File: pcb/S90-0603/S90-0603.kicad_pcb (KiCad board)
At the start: 2 copper layers, 100 x 40 mm, 9 parts

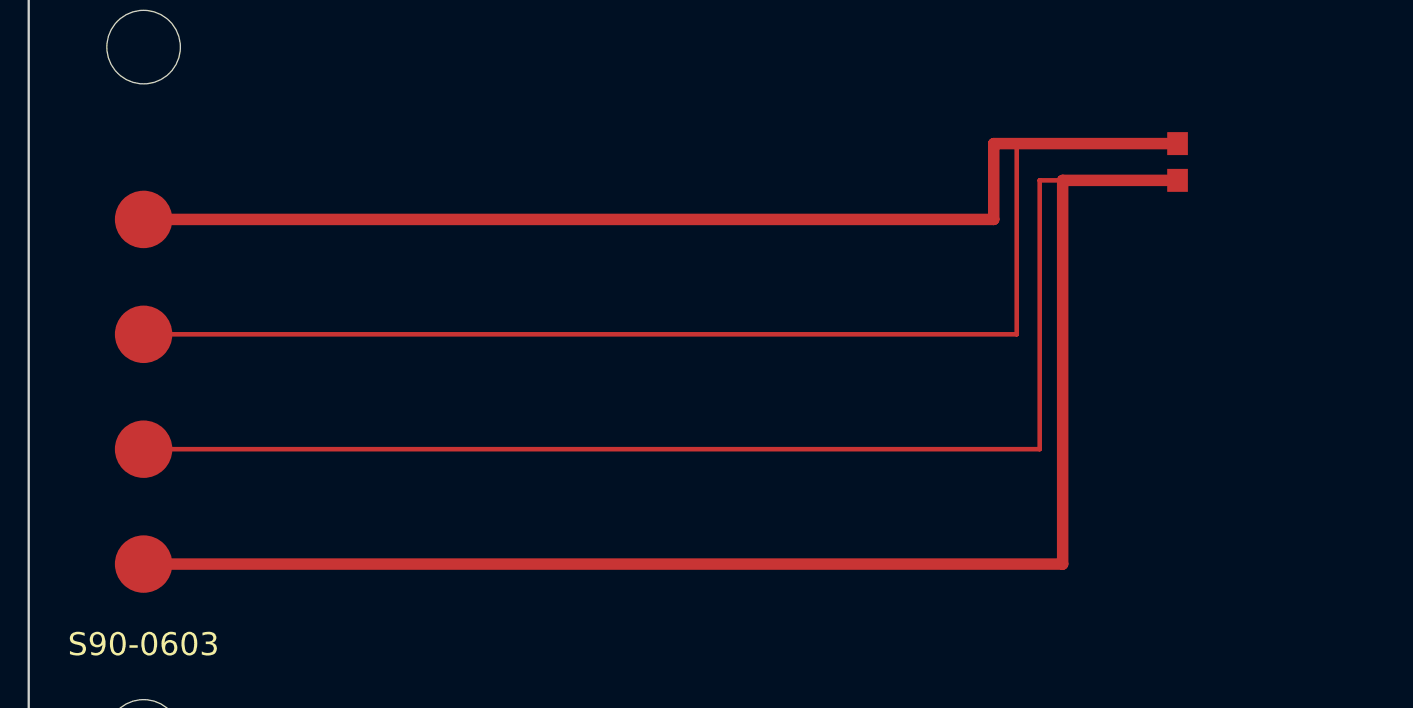
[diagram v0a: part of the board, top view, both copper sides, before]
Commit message: v0.3.1 — PCB CAD & JLCPCB Fabrication Package
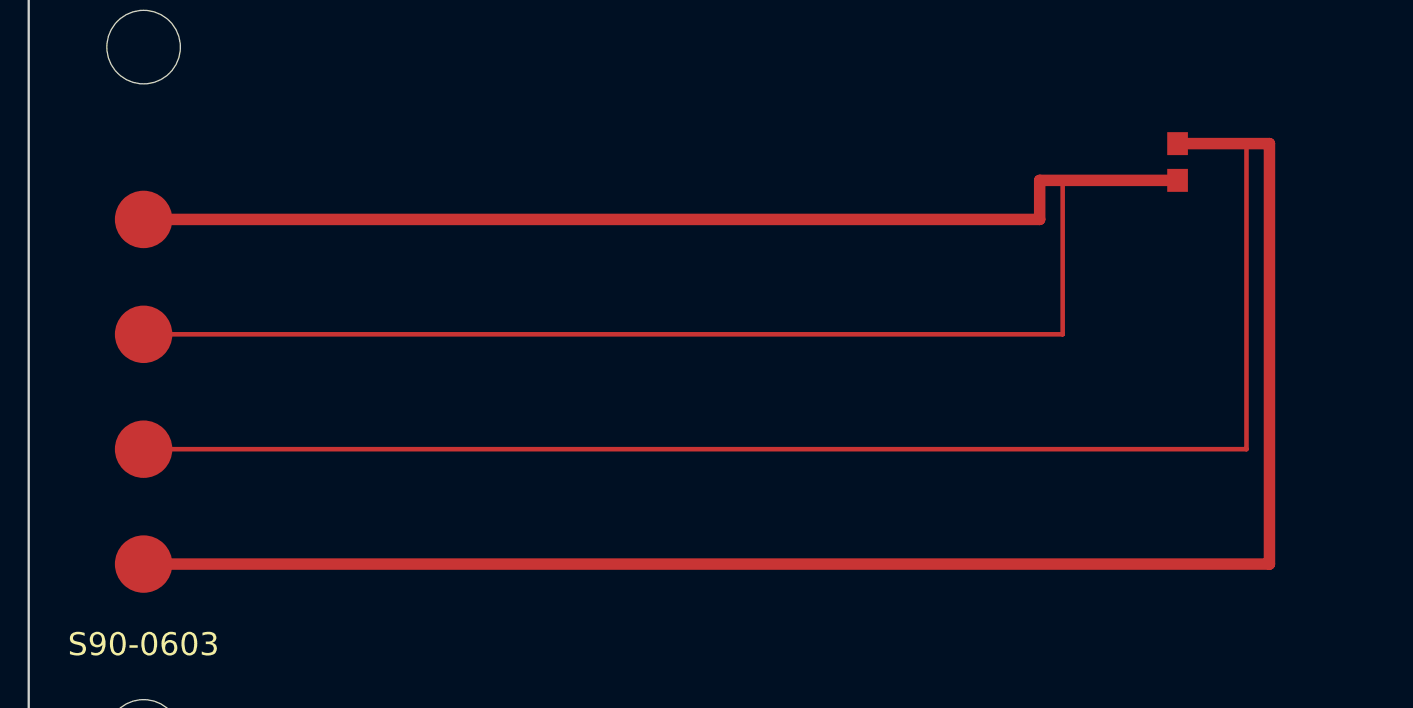
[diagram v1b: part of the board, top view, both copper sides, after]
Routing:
- net DRIVE_SENSE_MINUS: track 118.4 -> 135.6 mm
- net DRIVE_SENSE_PLUS: track 101.6 -> 98.4 mm
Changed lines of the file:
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@@
 		(pad "1" smd rect (at -0.8 0) (size 0.9 1.0) (layers "F.Cu" "F.Paste" "F.Mask") (net 1 "DRIVE_SENSE_PLUS"))
 		(pad "2" smd rect (at 0.8 0) (size 0.9 1.0) (layers "F.Cu" "F.Paste" "F.Mask") (net 2 "DRIVE_SENSE_MINUS"))
+		(model "/Applications/KiCad/KiCad.app/Contents/SharedSupport/3dmodels/Capacitor_SMD.3dshapes/C_0603_1608Metric.step"
+			(offset (xyz 0 0 0))
+			(scale (xyz 1 1 1))
+			(rotate (xyz 0 0 0))
+		)
 	)
 	(footprint "SC4:EdgeContact_2.5mm_Round" (layer "F.Cu")
@@
 		(pad "1" smd circle (at 0 0) (size 2.5 2.5) (layers "F.Cu" "F.Mask") (net 2 "DRIVE_SENSE_MINUS"))
 	)
-	(segment (start 5.0 12.5) (end 42.0 12.5) (width 0.5) (layer "F.Cu") (net 1))
-	(segment (start 42.0 12.5) (end 42.0 9.2) (width 0.5) (layer "F.Cu") (net 1))
-	(segment (start 42.0 9.2) (end 50.0 9.2) (width 0.5) (layer "F.Cu") (net 1))
-	(segment (start 5.0 17.5) (end 43.0 17.5) (width 0.2) (layer "F.Cu") (net 1))
-	(segment (start 43.0 17.5) (end 43.0 9.2) (width 0.2) (layer "F.Cu") (net 1))
-	(segment (start 43.0 9.2) (end 50.0 9.2) (width 0.2) (layer "F.Cu") (net 1))
-	(segment (start 5.0 22.5) (end 44.0 22.5) (width 0.2) (layer "F.Cu") (net 2))
-	(segment (start 44.0 22.5) (end 44.0 10.8) (width 0.2) (layer "F.Cu") (net 2))
-	(segment (start 44.0 10.8) (end 50.0 10.8) (width 0.2) (layer "F.Cu") (net 2))
-	(segment (start 5.0 27.5) (end 45.0 27.5) (width 0.5) (layer "F.Cu") (net 2))
-	(segment (start 45.0 27.5) (end 45.0 10.8) (width 0.5) (layer "F.Cu") (net 2))
-	(segment (start 45.0 10.8) (end 50.0 10.8) (width 0.5) (layer "F.Cu") (net 2))
+	(segment (start 5.0 12.5) (end 44.0 12.5) (width 0.5) (layer "F.Cu") (net 1))
+	(segment (start 44.0 12.5) (end 44.0 10.8) (width 0.5) (layer "F.Cu") (net 1))
+	(segment (start 44.0 10.8) (end 50.0 10.8) (width 0.5) (layer "F.Cu") (net 1))
+	(segment (start 5.0 17.5) (end 45.0 17.5) (width 0.2) (layer "F.Cu") (net 1))
+	(segment (start 45.0 17.5) (end 45.0 10.8) (width 0.2) (layer "F.Cu") (net 1))
+	(segment (start 45.0 10.8) (end 50.0 10.8) (width 0.2) (layer "F.Cu") (net 1))
+	(segment (start 5.0 22.5) (end 53.0 22.5) (width 0.2) (layer "F.Cu") (net 2))
+	(segment (start 53.0 22.5) (end 53.0 9.2) (width 0.2) (layer "F.Cu") (net 2))
+	(segment (start 53.0 9.2) (end 50.0 9.2) (width 0.2) (layer "F.Cu") (net 2))
+	(segment (start 5.0 27.5) (end 54.0 27.5) (width 0.5) (layer "F.Cu") (net 2))
+	(segment (start 54.0 27.5) (end 54.0 9.2) (width 0.5) (layer "F.Cu") (net 2))
+	(segment (start 54.0 9.2) (end 50.0 9.2) (width 0.5) (layer "F.Cu") (net 2))
 	(gr_text "S90-0603" (at 5.0 31.0 0) (layer "F.SilkS")
 		(effects (font (size 1 1) (thickness 0.15)))
